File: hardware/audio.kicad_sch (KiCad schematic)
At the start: 5 parts, among them J10 AudioJack_PJ-342

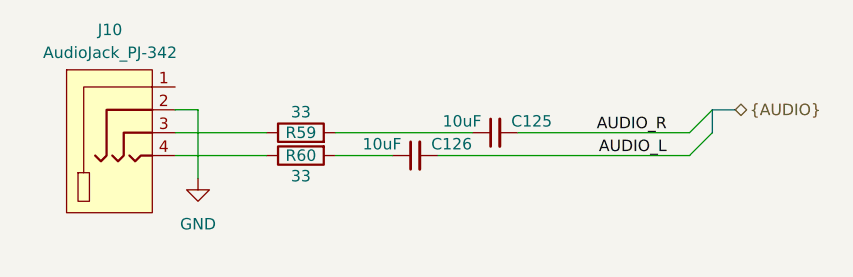
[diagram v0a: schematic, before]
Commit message: Finished with V1!
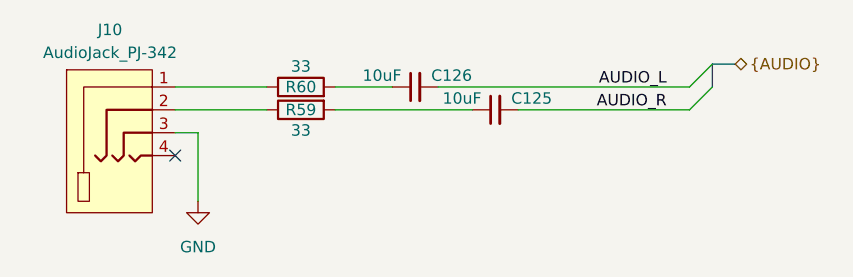
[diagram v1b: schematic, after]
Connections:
- net GND: now also J10.3; no longer J10.2
- net at J10.1: now also R60.1
- new net: J10.2, R59.1
- now unconnected: J10.4
- no-connect marks 0 -> 1
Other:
- moved on the sheet: C125, C126, R59, R60
